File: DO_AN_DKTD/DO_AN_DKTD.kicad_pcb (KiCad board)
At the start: 2 copper layers, 90.2 x 65.7 mm, 62 parts, among them J1 Conn_01x03, J2 Conn_01x02, J3 Conn_01x07, J4 Conn_01x04, J5 Conn_01x02, Q1 NPN, Q2 NPN, Q3 NPN, Q4 NPN, SW2 RotaryEncoder_Switch, U1 AMS1117, U2 74HC595, U3 MOC3020M, U4 PC817, U5 DevKitSTM32

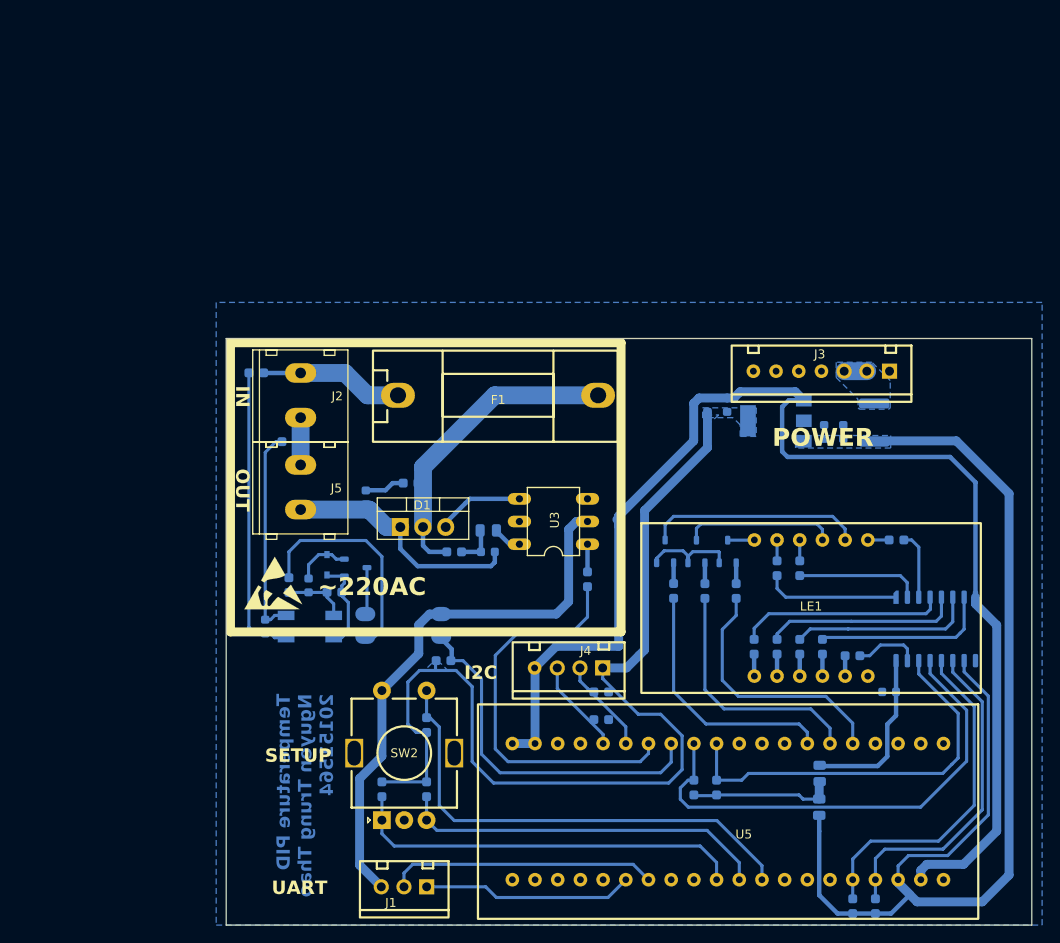
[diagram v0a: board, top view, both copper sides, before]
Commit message: completed layout PCB Ver 1.0
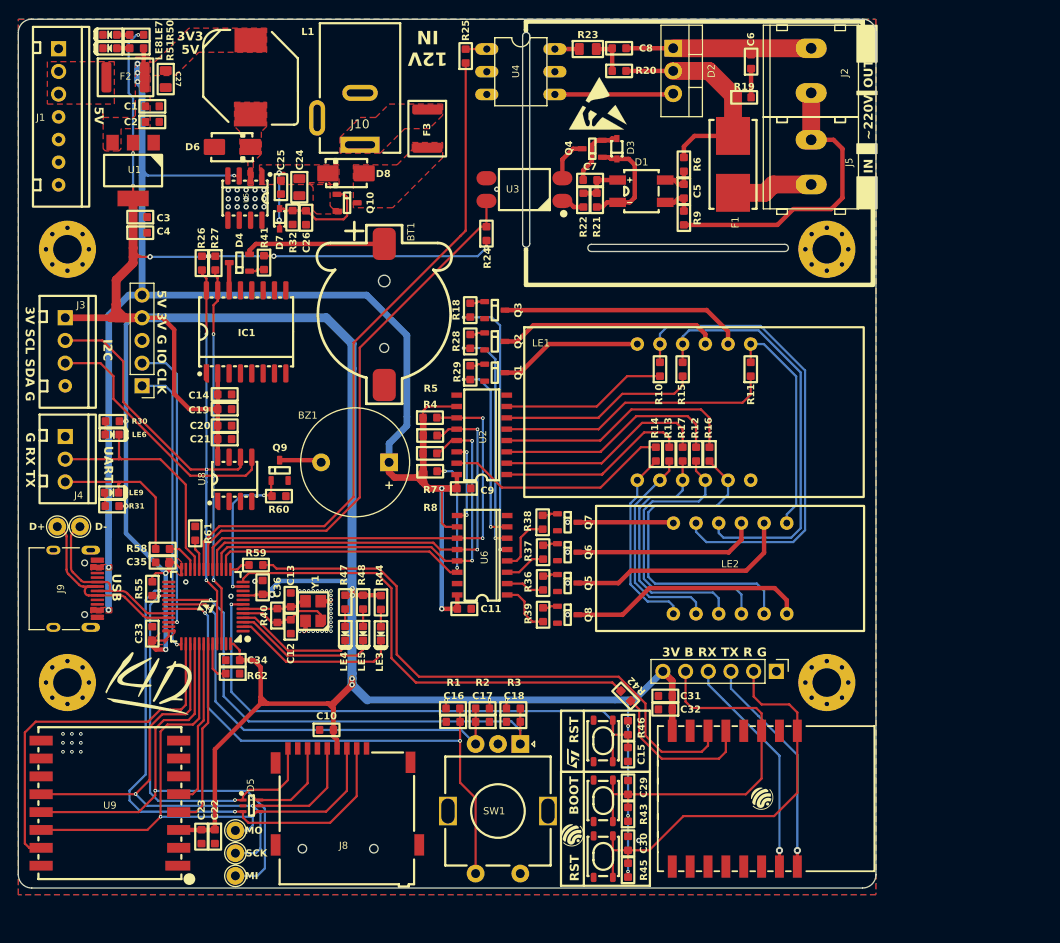
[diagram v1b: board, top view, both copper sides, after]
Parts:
- added BT1: CR1220, IVS_FOOTPRINTS:BatteryHolder_CR1220, F.Cu at (137.0, 80.0)
- added BZ1: Buzzer, Buzzer_Beeper:Buzzer_12x9.5RM7.6, F.Cu at (137.5, 96.6)
- added C10: 100nF, IVS_FOOTPRINTS:C_0603, F.Cu at (130.5, 126.5)
- added C11: 100nF, IVS_FOOTPRINTS:C_0603, F.Cu at (145.9, 113.0)
- added C12: 22pF, IVS_FOOTPRINTS:C_0603, F.Cu at (126.5, 115.0)
- added C13: 22pF, IVS_FOOTPRINTS:C_0603, F.Cu at (126.5, 112.0)
- added C14: 10uF, IVS_FOOTPRINTS:C_0603, F.Cu at (119.1, 89.0)
- added C15: 1uF, IVS_FOOTPRINTS:C_0603, F.Cu at (164.2, 129.3)
- added C16: 1uF, IVS_FOOTPRINTS:C_0603, F.Cu at (144.7, 125.7)
- added C17: 1uF, IVS_FOOTPRINTS:C_0603, F.Cu at (148.0, 125.7)
- added C18: 1uF, IVS_FOOTPRINTS:C_0603, F.Cu at (151.4, 125.7)
- added C19: 100nF, IVS_FOOTPRINTS:C_0603, F.Cu at (119.1, 90.7)
- added C20: 10uF, IVS_FOOTPRINTS:C_0603, F.Cu at (119.1, 92.5)
- added C21: 100nF, IVS_FOOTPRINTS:C_0603, F.Cu at (119.1, 94.0)
- added C22: 1uF, IVS_FOOTPRINTS:C_0603, F.Cu at (118.0, 138.5)
- added C23: 100nF, IVS_FOOTPRINTS:C_0603, F.Cu at (116.5, 138.5)
- added C24: 10uF, IVS_FOOTPRINTS:C_0805, F.Cu at (127.5, 65.8)
- added C25: 1uF, IVS_FOOTPRINTS:C_0603, F.Cu at (125.4, 65.8)
- added C26: 100nF, IVS_FOOTPRINTS:C_0603, F.Cu at (128.2, 69.2)
- added C27: 10uF, IVS_FOOTPRINTS:C_0805, F.Cu at (112.5, 53.7)
- added C29: 1uF, IVS_FOOTPRINTS:C_0603, F.Cu at (164.2, 133.0)
- added C30: 1uF, IVS_FOOTPRINTS:C_0603, F.Cu at (164.2, 139.2)
- added C31: 1uF, IVS_FOOTPRINTS:C_0603, F.Cu at (168.4, 122.8)
- added C32: 100nF, IVS_FOOTPRINTS:C_0603, F.Cu at (168.4, 124.2)
- added C33: 100nF, IVS_FOOTPRINTS:C_0603, F.Cu at (111.0, 115.8)
- added C34: 100nF, IVS_FOOTPRINTS:C_0603, F.Cu at (120.0, 118.8)
- added C35: 100nF, IVS_FOOTPRINTS:C_0603, F.Cu at (112.2, 107.8)
- added C36: 100nF, IVS_FOOTPRINTS:C_0603, F.Cu at (123.3, 110.6)
- added D+: TestPoint, TestPoint:TestPoint_THTPad_D2.0mm_Drill1.0mm, F.Cu at (100.4, 103.8)
- added D-: TestPoint, TestPoint:TestPoint_THTPad_D2.0mm_Drill1.0mm, F.Cu at (102.9, 103.8)
- added D4: BAT54C, IVS_FOOTPRINTS:SOT23-3, F.Cu at (120.8, 74.2)
- added D5: SMF05C, IVS_FOOTPRINTS:TSSOP-6, F.Cu at (122.1, 135.1)
- added D6: SS54, IVS_FOOTPRINTS:D_SMA, F.Cu at (120.0, 61.3)
- added D7: D_Schottky, IVS_FOOTPRINTS:D_SOD323, F.Cu at (125.2, 69.3)
- added D8: SS54, IVS_FOOTPRINTS:D_SMA, F.Cu at (132.6, 64.2)
- added F3: Fuse, IVS_FOOTPRINTS:Fuse_1812_4532Metric, F.Cu at (141.8, 59.2)
- added G***: LOGO, IVS_FOOTPRINTS:LoGo_ST_2.5x1.5mm, F.Cu at (158.1, 129.8)
- added G***: LOGO, IVS_FOOTPRINTS:LoGo_IDF_2.5x2.5mm, F.Cu at (158.1, 138.3)
- added G***: LOGO, IVS_FOOTPRINTS:LoGo_1412_10x8mm, F.Cu at (110.6, 121.7)
- added G***: LOGO, IVS_FOOTPRINTS:LoGo_ST_2.5x1.5mm, F.Cu at (117.0, 112.8)
- added G***: LOGO, IVS_FOOTPRINTS:LoGo_IDF_2.5x2.5mm, F.Cu at (179.3, 134.3)
- added G***: LOGO, IVS_FOOTPRINTS:LoGo_1412_10x8mm, B.Cu at (164.6, 68.3)
- added IC1: RTC_DS3231M, IVS_FOOTPRINTS:SOIC-16W_7.5x10.3mm_P1.27mm, F.Cu at (121.5, 82.0)
- added J10: Jack-DC, IVS_FOOTPRINTS:BarrelJack_Wuerth_6941xx301002, F.Cu at (134.2, 55.2)
- added J6: , Connector_PinHeader_2.54mm:PinHeader_1x06_P2.54mm_Vertical, F.Cu at (180.8, 120.0)
- added J7: Conn_01x05_Male, Connector_PinHeader_2.54mm:PinHeader_1x05_P2.54mm_Vertical, F.Cu at (109.8, 88.0)
- added J8: Micro_SD_Card_Det1, IVS_FOOTPRINTS:MicroSD_Socket_9P, F.Cu at (132.4, 139.8)
- added J9: USB_C_Receptacle, IVS_FOOTPRINTS:USB_C_Receptacle_XKB_U262-16XN-4BVC11, F.Cu at (101.0, 110.8)
- added L1: 68uH 2A, IVS_FOOTPRINTS:L_10.4x10.4_H4.8, F.Cu at (122.0, 53.5)
- added LE2: 5631AS, IVS_FOOTPRINTS:7Segment_4led_Cathode_30x14mm, F.Cu at (175.7, 108.5)
- added LE3: Led, IVS_FOOTPRINTS:LED_0603, F.Cu at (136.6, 115.8)
- added LE4: Led, IVS_FOOTPRINTS:LED_0603, F.Cu at (132.6, 115.8)
- added LE5: Led, IVS_FOOTPRINTS:LED_0603, F.Cu at (134.6, 115.8)
- added LE6: Led, IVS_FOOTPRINTS:LED_0603, F.Cu at (106.5, 93.5)
- added LE7: Led, IVS_FOOTPRINTS:LED_0603, F.Cu at (106.2, 48.8)
- added LE8: Led, IVS_FOOTPRINTS:LED_0603, F.Cu at (106.2, 50.2)
- added LE9: Led, IVS_FOOTPRINTS:LED_0603, F.Cu at (106.5, 100.0)
- added MI: TestPoint, TestPoint:TestPoint_THTPad_D2.0mm_Drill1.0mm, F.Cu at (120.3, 142.9)
- added MO: TestPoint, TestPoint:TestPoint_THTPad_D2.0mm_Drill1.0mm, F.Cu at (120.3, 137.8)
- added Q10: P_Mosfet, IVS_FOOTPRINTS:SOT23-3, F.Cu at (132.8, 67.5)
- added Q5: NPN, IVS_FOOTPRINTS:SOT23-3, F.Cu at (157.5, 110.1)
- added Q6: NPN, IVS_FOOTPRINTS:SOT23-3, F.Cu at (157.5, 106.7)
- added Q7: NPN, IVS_FOOTPRINTS:SOT23-3, F.Cu at (157.5, 103.3)
- added Q8: NPN, IVS_FOOTPRINTS:SOT23-3, F.Cu at (157.5, 113.7)
- added Q9: N_Mosfet, IVS_FOOTPRINTS:SOT23-3, F.Cu at (125.2, 97.5)
- added R32: 12k, IVS_FOOTPRINTS:R_0603, F.Cu at (126.7, 69.2)
- added R36: 2k, IVS_FOOTPRINTS:R_0603, F.Cu at (154.7, 110.1)
- added R37: 2k, IVS_FOOTPRINTS:R_0603, F.Cu at (154.7, 106.7)
- added R38: 2k, IVS_FOOTPRINTS:R_0603, F.Cu at (154.7, 103.3)
- added R39: 2k, IVS_FOOTPRINTS:R_0603, F.Cu at (154.7, 113.7)
- added R40: 1M, IVS_FOOTPRINTS:R_0603, F.Cu at (125.0, 113.8)
- added R41: 1k, IVS_FOOTPRINTS:R_0603, F.Cu at (123.5, 74.2)
- added R42: 100, IVS_FOOTPRINTS:R_0603, F.Cu at (164.0, 122.8)
- added R43: 10k, IVS_FOOTPRINTS:R_0603, F.Cu at (164.2, 136.0)
- added R44: 1k, IVS_FOOTPRINTS:R_0603, F.Cu at (136.6, 112.3)
- added R45: 10k, IVS_FOOTPRINTS:R_0603, F.Cu at (164.2, 142.2)
- added R46: 10k, IVS_FOOTPRINTS:R_0603, F.Cu at (164.2, 126.3)
- added R47: 1k, IVS_FOOTPRINTS:R_0603, F.Cu at (132.6, 112.2)
- added R48: 1k, IVS_FOOTPRINTS:R_0603, F.Cu at (134.6, 112.2)
- added R50: 1k, IVS_FOOTPRINTS:R_0603, F.Cu at (109.2, 48.8)
- added R51: 1k, IVS_FOOTPRINTS:R_0603, F.Cu at (109.2, 50.2)
- added R55: 4k7, IVS_FOOTPRINTS:R_0603, F.Cu at (111.0, 110.8)
- added R58: 100R, IVS_FOOTPRINTS:R_0603, F.Cu at (112.2, 106.3)
- added R59: 100R, IVS_FOOTPRINTS:R_0603, F.Cu at (122.6, 108.1)
- added R60: 1M, IVS_FOOTPRINTS:R_0603, F.Cu at (125.2, 100.4)
- added R61: 10K, IVS_FOOTPRINTS:R_0603, F.Cu at (115.8, 104.5)
- added R62: 10K, IVS_FOOTPRINTS:R_0603, F.Cu at (120.0, 120.2)
- added REF**: MountingHole_3.2mm_M3_Pad_Via, MountingHole:MountingHole_3.2mm_M3_Pad_Via, F.Cu at (186.5, 121.2)
- added REF**: MountingHole_3.2mm_M3_Pad_Via, MountingHole:MountingHole_3.2mm_M3_Pad_Via, F.Cu at (186.5, 72.8)
- added REF**: MountingHole_3.2mm_M3_Pad_Via, MountingHole:MountingHole_3.2mm_M3_Pad_Via, F.Cu at (101.5, 121.2)
- added REF**: MountingHole_3.2mm_M3_Pad_Via, MountingHole:MountingHole_3.2mm_M3_Pad_Via, F.Cu at (101.5, 72.8)
- added SCK: TestPoint, TestPoint:TestPoint_THTPad_D2.0mm_Drill1.0mm, F.Cu at (120.3, 140.3)
- added SW1: RotaryEncoder_Switch, IVS_FOOTPRINTS:RotaryEncoder_Alps_EC11E-Switch_Vertical_H20mm, F.Cu at (149.8, 135.7)
- added SW3: SW_Push, IVS_FOOTPRINTS:SW_SPST_PTS810, F.Cu at (161.5, 134.5)
- added SW4: SW_Push, IVS_FOOTPRINTS:SW_SPST_PTS810, F.Cu at (161.5, 127.8)
- added U10: ESP-07, IVS_FOOTPRINTS:ESP8266-07__ESP32-C3-12F, F.Cu at (184.2, 126.1)
- added U6: 74HC595, IVS_FOOTPRINTS:SOIC-16W_3.92x10.2mm, F.Cu at (147.9, 107.0)
- added U7: STM32F103C8Tx, IVS_FOOTPRINTS:LQFP-48_7x7mm_P0.5mm, F.Cu at (117.0, 112.8)
- added U8: 24C32N, IVS_FOOTPRINTS:SOIC-8_3.9x4.9mm_P1.27mm, F.Cu at (120.2, 98.5)
- added U9: Ai-Thinker-Ra-02, IVS_FOOTPRINTS:MODULE_RA-02_LORA, F.Cu at (106.2, 134.8)
- added Y1: Crystal_GND24_Small, IVS_FOOTPRINTS:Crystal_3225_4P_3.2x2.6mm, F.Cu at (129.0, 113.2)
- C1: value 100nF -> 1uF; moved to F.Cu
- C2: value 1uF -> 100nF; moved to F.Cu
- C3, C4, C6, C9, D3, F2, Q1, Q2, Q3, Q4, U1: moved to F.Cu
- C5: value 50nF -> 10nF; moved to F.Cu
- C7: value 10nF -> 10uF; moved to F.Cu
- C8: value 10uF -> 50nF; moved to F.Cu
- D1: value TRIAC -> MB10F; footprint IVS_FOOTPRINTS:TO-220-3_Vertical -> IVS_FOOTPRINTS:Bridge_MB10F-13
- D2: value MB10F -> TRIAC; footprint IVS_FOOTPRINTS:Bridge_MB10F-13 -> IVS_FOOTPRINTS:TO-220-3_Vertical; moved to F.Cu
- F1: footprint IVS_FOOTPRINTS:Fuse_BLX-A-P22.4mm -> IVS_FOOTPRINTS:Fuseholder_Littelfuse_Nano2_154x
- J1: value Conn_01x03 -> Conn_01x07; footprint IVS_FOOTPRINTS:Conn_XH-P2.54mm-3P -> IVS_FOOTPRINTS:Conn_XH-P2.54mm-7P
- J3: value Conn_01x07 -> Conn_01x04; footprint IVS_FOOTPRINTS:Conn_XH-P2.54mm-7P -> IVS_FOOTPRINTS:Conn_XH-P2.54mm-4P
- J4: value Conn_01x04 -> Conn_01x03; footprint IVS_FOOTPRINTS:Conn_XH-P2.54mm-4P -> IVS_FOOTPRINTS:Conn_XH-P2.54mm-3P
- R1, R10, R11, R2, R20, R3: footprint IVS_FOOTPRINTS:R0603 -> IVS_FOOTPRINTS:R_0603; moved to F.Cu
- R12, R13, R14: value 2k -> 1k; footprint IVS_FOOTPRINTS:R0603 -> IVS_FOOTPRINTS:R_0603; moved to F.Cu
- R15, R16, R17, R30, R31: value 4k7 -> 1k; footprint IVS_FOOTPRINTS:R0603 -> IVS_FOOTPRINTS:R_0603; moved to F.Cu
- R18: value 4k7 -> 2k; footprint IVS_FOOTPRINTS:R0603 -> IVS_FOOTPRINTS:R_0603; moved to F.Cu
- R19: value 360 -> 39; footprint IVS_FOOTPRINTS:R0805 -> IVS_FOOTPRINTS:R_0603; moved to F.Cu
- R21: value 39 -> 22k; footprint IVS_FOOTPRINTS:R0603 -> IVS_FOOTPRINTS:R_0603; moved to F.Cu
- R22: value 360 -> 1k; footprint IVS_FOOTPRINTS:R0603 -> IVS_FOOTPRINTS:R_0603; moved to F.Cu
- R23: value 180k -> 360; footprint IVS_FOOTPRINTS:R0603 -> IVS_FOOTPRINTS:R_0805; moved to F.Cu
- R24: value 180k -> 1k; footprint IVS_FOOTPRINTS:R0603 -> IVS_FOOTPRINTS:R_0603; moved to F.Cu
- R25: value 1k -> 360; footprint IVS_FOOTPRINTS:R0603 -> IVS_FOOTPRINTS:R_0603; moved to F.Cu
- R26: value 22k -> 4k7; footprint IVS_FOOTPRINTS:R0603 -> IVS_FOOTPRINTS:R_0603; moved to F.Cu
- R27, R4, R5, R7, R8: value 1k -> 4k7; footprint IVS_FOOTPRINTS:R0603 -> IVS_FOOTPRINTS:R_0603; moved to F.Cu
- R28, R29: value 0R -> 2k; footprint IVS_FOOTPRINTS:R0805 -> IVS_FOOTPRINTS:R_0603; moved to F.Cu
- R6, R9: value 1k -> 180k; footprint IVS_FOOTPRINTS:R0603 -> IVS_FOOTPRINTS:R_0603; moved to F.Cu
- SW2: value RotaryEncoder_Switch -> SW_Push; footprint IVS_FOOTPRINTS:RotaryEncoder_Alps_EC11E-Switch_Vertical_H20mm -> IVS_FOOTPRINTS:SW_SPST_PTS810
- U2: footprint IVS_FOOTPRINTS:SOIC-16W_5.3x10.2mm_P1.27mm -> IVS_FOOTPRINTS:SOIC-16W_3.92x10.2mm; moved to F.Cu
- U3: value MOC3020M -> PC817; footprint IVS_FOOTPRINTS:DIL06-E -> IVS_FOOTPRINTS:OPTO_SOT254P975X400-4N
- U4: value PC817 -> MOC3020M; footprint IVS_FOOTPRINTS:OPTO_SOT254P975X400-4N -> IVS_FOOTPRINTS:DIL06-E; moved to F.Cu
- U5: value DevKitSTM32 -> XL1509; footprint IVS_FOOTPRINTS:DevKitSTM32 -> IVS_FOOTPRINTS:SOIC-8_3.9x4.9mm_P1.27mm
- moved J1 94.5 mm to (100.5, 57.9), turned to 0 degrees
- moved F2 92.3 mm to (108.0, 53.5), turned to 0 degrees
- moved U5 88.2 mm to (121.4, 67.0)
- moved C2 84.8 mm to (111.0, 58.5), turned to 0 degrees
- moved J3 84.7 mm to (101.2, 84.2), turned to 0 degrees
- moved C1 83.6 mm to (111.0, 56.8), turned to 180 degrees
- moved U1 76.9 mm to (109.0, 64.0), turned to 180 degrees
- moved D2 76.4 mm to (169.3, 50.2), turned to -90 degrees
- moved C8 69.5 mm to (163.2, 50.2), turned to 0 degrees
- moved C4 68.5 mm to (109.7, 70.9), turned to 0 degrees
- moved J5 67.8 mm to (184.8, 63.0)
- moved J2 67.7 mm to (184.8, 52.8)
- moved C3 66.9 mm to (109.7, 69.2), turned to 180 degrees
- moved C6 65.1 mm to (178.0, 51.8), turned to 90 degrees
- moved REF** 64.8 mm to (160.9, 56.4)
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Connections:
- C1 pad 1: +5V -> GND
- C1 pad 2: GND -> +5V
- C2 pad 1: GND -> +5V
- C2 pad 2: +5V -> GND
- C5 pad 2: Net-(D1-A1) -> Net-(C5-Pad2)
- C6 pad 2: Net-(D1-A1) -> /Peripheral/Load
- C7 pad 1: Net-(C7-Pad1) -> Net-(D1-+)
- C7 pad 2: Net-(C7-Pad2) -> Net-(Q4-E)
- C8 pad 1: Net-(D2-+) -> Net-(C8-Pad1)
- C8 pad 2: Net-(Q4-E) -> /Peripheral/Load
- C9 pad 2: Net-(U2-VCC) -> +5V
- D1 pad 1: Net-(D1-A1) -> Net-(D1-+)
- D1 pad 2: Net-(D1-A2) -> Net-(C5-Pad2)
- D1 pad 3: Net-(D1-G) -> Net-(D1--)
- D2 pad 1: Net-(D2-+) -> /Peripheral/Load
- D2 pad 2: Net-(C7-Pad2) -> /Peripheral/L_after
- D2 pad 3: Net-(D2--) -> Net-(D2-G)
- D3 pad 2: Net-(D2--) -> Net-(D1--)
- F1 pad 1: Net-(D1-A2) -> /Peripheral/L_after
- F1 pad 2: /L -> /Peripheral/L
- F2 pad 1: /5vin -> /POWER/5vin
- J1 pad 1: /TX -> unconnected-(J1-Pin_1-Pad1)
- J1 pad 2: /RX -> /POWER/5vin
- J1 pad 3: GND -> /POWER/5vin
- J2 pad 1: /N -> /Peripheral/N
- J2 pad 2: /L -> /Peripheral/Load
- J3 pad 1: unconnected-(J3-Pin_1-Pad1) -> +3V3
- J3 pad 2: /5vin -> /Peripheral/24C32.SCL
- J3 pad 3: /5vin -> /Peripheral/24C32.SDA
- J4 pad 1: +3V3 -> GND
- J4 pad 2: /SCL -> /Peripheral/LOG_RX
- J4 pad 3: /SDA -> /Peripheral/LOG_TX
- J5 pad 1: Net-(D1-A1) -> /Peripheral/L
- J5 pad 2: /N -> /Peripheral/N
- Q4 pad 1: Net-(D2--) -> Net-(D1--)
- R1 pad 2: /EnC_B -> /Peripheral/Encoder.EnC_BT
- R10 pad 1: Net-(U2-QA) -> Net-(U2-QH)
- R10 pad 2: Net-(LE1-g) -> Net-(LE1-a)
- R11 pad 1: Net-(U2-QG) -> Net-(U2-QF)
- R11 pad 2: Net-(LE1-DPX) -> Net-(LE1-b)
- R12 pad 1: /LE1 -> Net-(U2-QD)
- R12 pad 2: Net-(Q3-B) -> Net-(LE1-c)
- R13 pad 1: /LE2 -> Net-(U2-QB)
- R13 pad 2: Net-(Q2-B) -> Net-(LE1-d)
- R14 pad 1: /LE3 -> Net-(U2-QA)
- R14 pad 2: Net-(Q1-B) -> Net-(LE1-e)
- R15 pad 1: Net-(R15-Pad1) -> Net-(U2-QG)
- R15 pad 2: /SER -> Net-(LE1-f)
- R16 pad 1: +5V -> Net-(U2-QE)
- R16 pad 2: /SRCLK -> Net-(LE1-g)
- R17 pad 1: +5V -> Net-(U2-QC)
- R17 pad 2: /RCLK -> Net-(LE1-DPX)
- R18 pad 1: Net-(R15-Pad1) -> /Peripheral/LE3
- R18 pad 2: /OE -> Net-(Q3-B)
- R19 pad 1: Net-(R19-Pad1) -> /Peripheral/L_after
- R19 pad 2: Net-(C5-Pad1) -> Net-(C6-Pad1)
- R2 pad 2: /EnC_A -> /Peripheral/Encoder.EnC_B
- R20 pad 1: Net-(C5-Pad1) -> Net-(C8-Pad1)
- R20 pad 2: Net-(D1-A2) -> /Peripheral/L_after
- R21 pad 1: Net-(D1-A2) -> Net-(D1-+)
- R21 pad 2: Net-(C6-Pad1) -> Net-(D1--)
- R22 pad 1: /TRIAC -> Net-(R22-Pad1)
- R22 pad 2: Net-(R22-Pad2) -> Net-(D1-+)
- R23 pad 1: Net-(C7-Pad1) -> Net-(R23-Pad1)
- R23 pad 2: /L -> Net-(C8-Pad1)
- R24 pad 1: Net-(C7-Pad2) -> +3V3
- R24 pad 2: /N -> /Peripheral/AC_DET
- R25 pad 1: Net-(R25-Pad1) -> /Peripheral/TRIAC
- R25 pad 2: Net-(D2-+) -> Net-(R25-Pad2)
- R26 pad 1: Net-(D2-+) -> +3V3
- R26 pad 2: Net-(D2--) -> /Peripheral/24C32.SCL
- R27 pad 2: /AC_DET -> /Peripheral/24C32.SDA
- R28 pad 1: Net-(U2-VCC) -> /Peripheral/LE2
- R28 pad 2: Net-(R15-Pad1) -> Net-(Q2-B)
- R29 pad 1: Net-(R15-Pad1) -> /Peripheral/LE1
- R29 pad 2: +5V -> Net-(Q1-B)
- R3 pad 2: /EnC_BT -> /Peripheral/Encoder.EnC_A
- R30 pad 2: /SCL -> Net-(LE6-Pad1)
- R31 pad 2: /SDA -> Net-(LE9-Pad1)
- R4 pad 1: Net-(U2-QB) -> +5V
- R4 pad 2: Net-(LE1-a) -> /Peripheral/74HC595.RCLK
- R5 pad 1: Net-(U2-QD) -> +5V
- R5 pad 2: Net-(LE1-b) -> /Peripheral/74HC595.SRCLK
- R6 pad 1: Net-(U2-QH) -> Net-(C5-Pad1)
- R6 pad 2: Net-(LE1-c) -> /Peripheral/L_after
- R7 pad 1: Net-(U2-QF) -> +5V
- R7 pad 2: Net-(LE1-d) -> /Peripheral/74HC595.OE
- R8 pad 1: Net-(U2-QE) -> +5V
- R8 pad 2: Net-(LE1-e) -> /Peripheral/74HC595.SER
- R9 pad 1: Net-(U2-QC) -> Net-(C5-Pad2)
- R9 pad 2: Net-(LE1-f) -> /Peripheral/N
- U2 pad 10: Net-(U2-VCC) -> +5V
- U2 pad 11: /SRCLK -> /Peripheral/74HC595.SRCLK
- U2 pad 12: /RCLK -> /Peripheral/74HC595.RCLK
- U2 pad 13: /OE -> /Peripheral/74HC595.OE
- U2 pad 14: /SER -> Net-(U2-SER)
- U2 pad 16: Net-(U2-VCC) -> +5V
- U3 pad 1: Net-(R22-Pad2) -> Net-(R22-Pad1)
- U3 pad 2: GND -> Net-(Q4-C)
- U3 pad 3: unconnected-(U3-NC-Pad3) -> GND
- U3 pad 4: Net-(D1-G) -> /Peripheral/AC_DET
- U4 pad 1: Net-(R25-Pad1) -> Net-(R25-Pad2)
- U4 pad 2: Net-(Q4-C) -> GND
- U4 pad 3: GND -> unconnected-(U4-NC-Pad3)
- U4 pad 4: /AC_DET -> Net-(D2-G)
- U5 pad 1: unconnected-(U5-VBAT-Pad1) -> VDC
- U5 pad 2: unconnected-(U5-PC13-Pad2) -> /POWER/VOUT
- U5 pad 3: unconnected-(U5-PC14-Pad3) -> +5V
- U5 pad 4: unconnected-(U5-PC15-Pad4) -> GND
- U5 pad 5: /LE3 -> GND
- U5 pad 6: /LE2 -> GND
- U5 pad 7: /LE1 -> GND
- U5 pad 8: unconnected-(U5-PA3-Pad8) -> GND
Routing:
- net +3V3: track 112.5 -> 368.7 mm, vias 0 -> 22
- net GND: track 220.8 -> 2.42 mm, vias 0 -> 57
- net /Peripheral/TRIAC: track 0.00 -> 75.7 mm
- net /Peripheral/24C32.SCL: track 0.00 -> 72.8 mm, vias 0 -> 3
- net /Peripheral/24C32.SDA: track 0.00 -> 71.8 mm, vias 0 -> 3
- net /Peripheral/LORA.MISO: track 0.00 -> 68.3 mm, vias 0 -> 2
- net /ESP/TX_ESP32: track 0.00 -> 67.0 mm
- net /Peripheral/LORA.MOSI: track 0.00 -> 66.9 mm, vias 0 -> 2
- net /Peripheral/LORA.SCK: track 0.00 -> 66.9 mm, vias 0 -> 2
- net /STM32/RST: track 0.00 -> 64.5 mm, vias 0 -> 2
- net /Peripheral/Encoder.EnC_BT: track 0.00 -> 64.0 mm, vias 0 -> 2
- net /Peripheral/AC_DET: track 0.00 -> 61.4 mm
- net /Peripheral/SD.CS: track 0.00 -> 59.6 mm, vias 0 -> 2
- net /Peripheral/Encoder.EnC_A: track 0.00 -> 56.4 mm, vias 0 -> 1
- net /OE: track 54.7 -> 0.00 mm
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- added copper zone on F.Cu, net +3V3
- added copper zone on F.Cu, net +5V
- added copper zone on F.Cu, net /POWER/5vin
- added copper zone on F.Cu, net /POWER/A
- added copper zone on F.Cu, net /POWER/B
- added copper zone on F.Cu, net /POWER/VOUT
- added copper zone on F.Cu, net GND
- added copper zone on F.Cu, net VDC
- removed copper zone on B.Cu, net +3V3
- removed copper zone on B.Cu, net +5V
- removed copper zone on B.Cu, net /5vin
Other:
- board size 90.2 x 65.7 mm -> 96 x 97.2 mm
- board text added: "12V IN"
- board text added: "3V B RX TX R G"
- board text added: "3V SCL SDA G"
- board text added: "3V3"
- board text added: "5V"
- board text added: "5V 3V G IO CLK"
- board text added: "BOOT"
- board text added: "BORAD V0.1 Designed By Nguyen Trung Thao 20151564"
- board text added: "G RX TX"
- board text added: "RST"
- board text added: "USB"
- board text added: "~220V"
- board text removed: "POWER"
- board text removed: "SETUP"
- board text removed: "Temperature PID Nguyen Trung Thao 20151564"
- board text removed: "~220AC"
